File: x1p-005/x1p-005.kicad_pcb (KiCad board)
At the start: 2 copper layers, 26 x 61.8 mm, 72 parts, among them Q1 LMBT3904LT1G, SW1 6.0*6.0*6.0, SW2 6.0*6.0*6.0, U1 AD24C02, U2 SN74LVC1T45DBVR, U4 SN74LVC1G3157DBVR_C3040658, U5 SN74LVC1G3157DBVR_C3040658

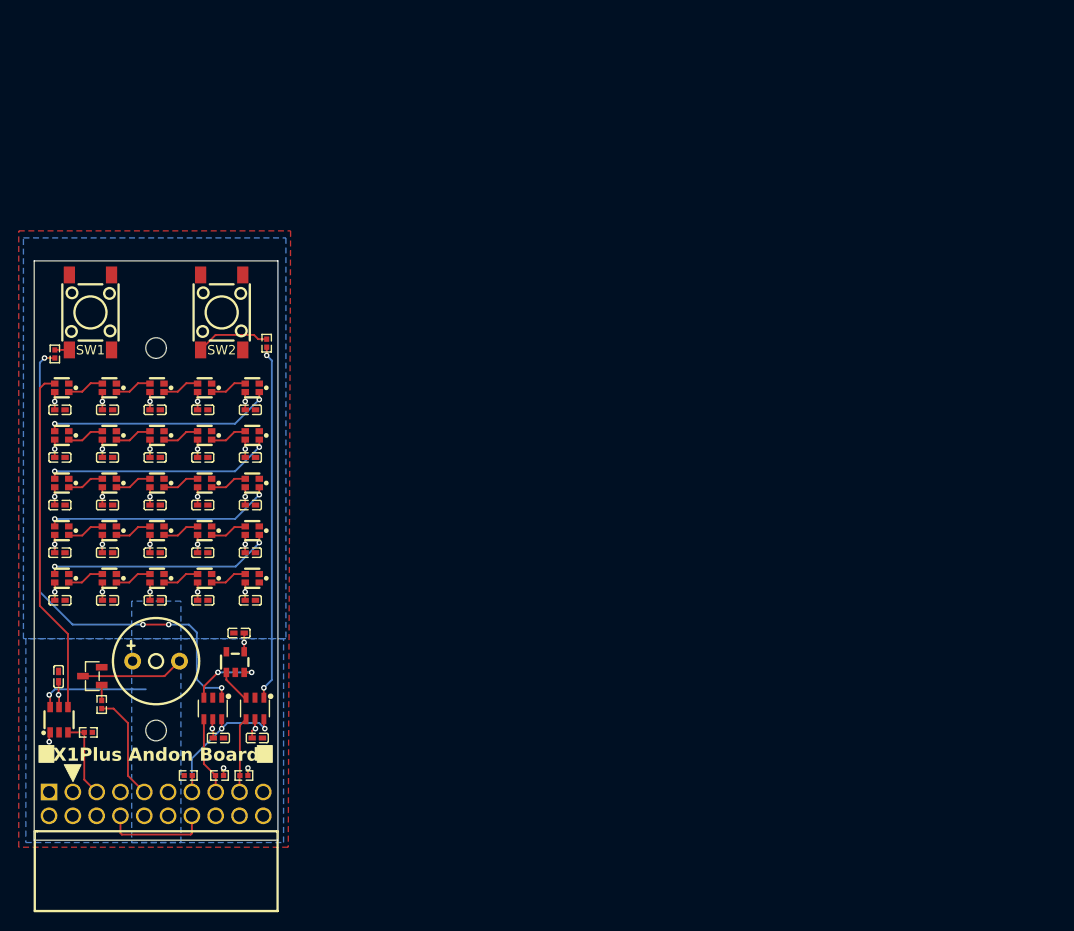
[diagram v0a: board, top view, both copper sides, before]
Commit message: x1p-005: fix up board layout to align with x1p-004
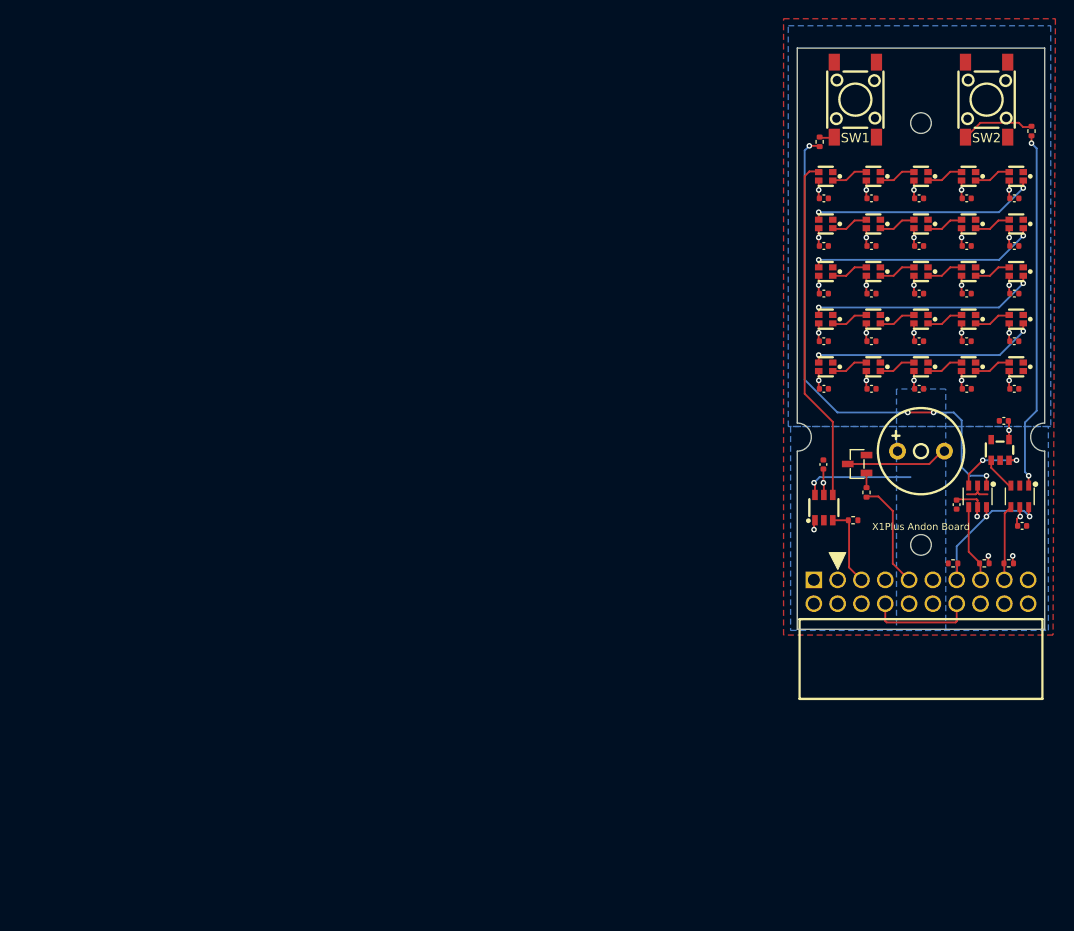
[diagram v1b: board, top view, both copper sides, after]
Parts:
- C1, C13, C14: footprint x1p-005:C0402 -> Capacitor_SMD:C_0402_1005Metric
- C10, C11, C12, C15, C16, C17, C18, C19, C2, C20, C21, C22, C23, C24, C25, C26, C27, C28, C29, C3, C4, C5, C6, C7, C8, C9: footprint x1p-004:C0402 -> Capacitor_SMD:C_0402_1005Metric
- R1, R2, R3, R4, R5, R6, R7: footprint x1p-005:R0402 -> Resistor_SMD:R_0402_1005Metric
- moved H1 85.1 mm to (150.0, 50.0)
- moved SW1 84.7 mm to (143.0, 47.5)
- moved SW2 84.7 mm to (157.0, 47.5)
- moved R2 84.7 mm to (159.4, 97.0)
- moved C1 84.7 mm to (158.8, 81.8)
- moved C2 84.7 mm to (139.6, 86.4)
- moved HDR1 84.7 mm to (150.0, 100.0)
- moved Q1 84.7 mm to (143.2, 86.4)
- moved R4 84.7 mm to (139.2, 52.0)
- moved R6 84.7 mm to (144.2, 89.4)
- moved U1 84.7 mm to (158.4, 84.9)
- moved C14 84.7 mm to (160.8, 93.0)
- moved R1 84.7 mm to (156.8, 97.0)
- moved R3 84.7 mm to (142.8, 92.4)
- moved R5 84.7 mm to (153.4, 97.0)
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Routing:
- net GND: track 0.00 -> 3.10 mm
- net 3V3: track 23.5 -> 25.6 mm
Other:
- board size 26 x 61.8 mm -> 26.4 x 62 mm
- board text added: "X1P-005-B02"
- board text removed: "X1P-005-B01"
